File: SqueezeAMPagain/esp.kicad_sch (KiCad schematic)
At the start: 12 parts, among them J3 Conn_ARM_JTAG_SWD_10, U2 ESP32-WROVER-E

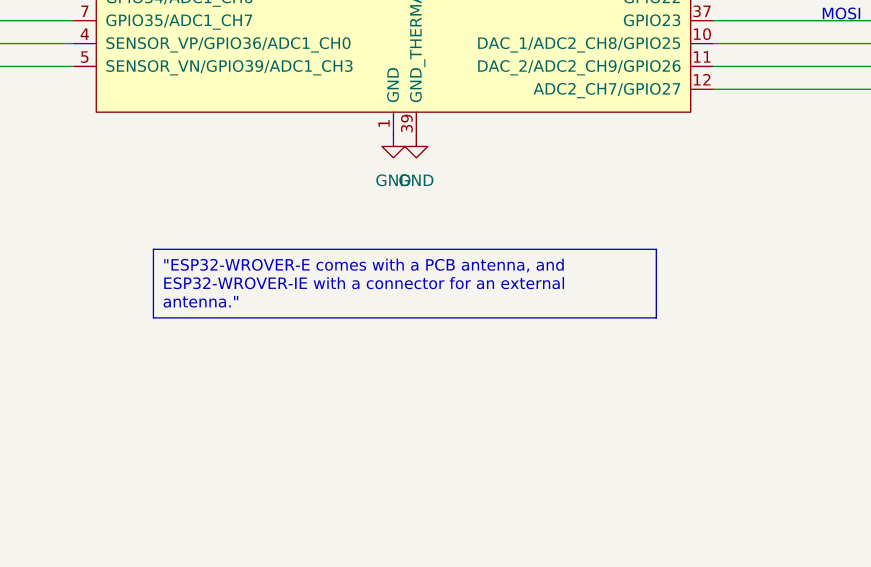
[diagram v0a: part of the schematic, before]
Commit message: v2
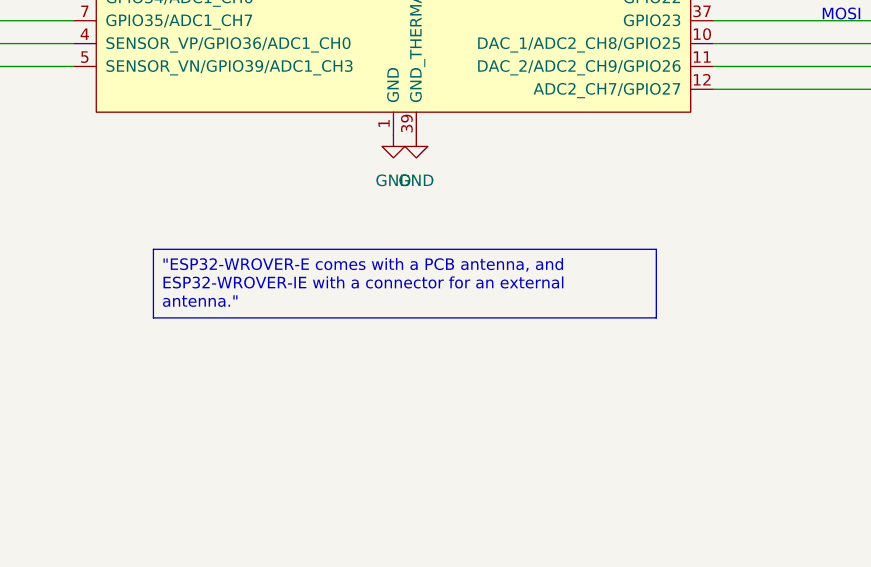
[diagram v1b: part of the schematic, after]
